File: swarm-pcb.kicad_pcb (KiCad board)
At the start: 4 copper layers, 45 x 40 mm, 120 parts, among them Q301 CJ3139K, U101 USB-TYPE-C-018, U102 2450AT18A100E, U103 ESP32-S3, U104 TS-1187A-B-A-B, U105 TS-1187A-B-A-B, U201 A3901SEJTR-T, U202 ICM-42670-P, U203 NH-B1515RGBA-HF, U205 Motor_1, U206 Motor_2, U301 TLV62569DRL, U302 TP4065, U303 BATT, X101 TZ1269D

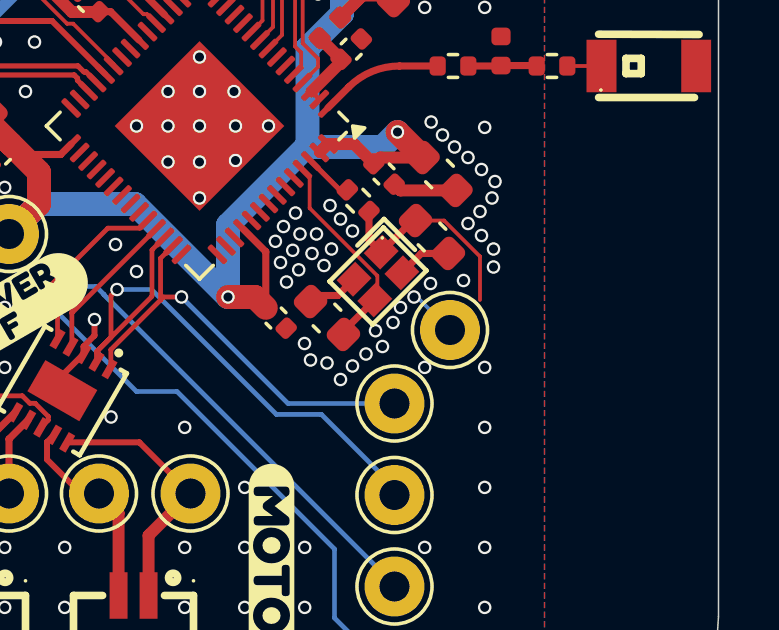
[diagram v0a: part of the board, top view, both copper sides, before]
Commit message: production
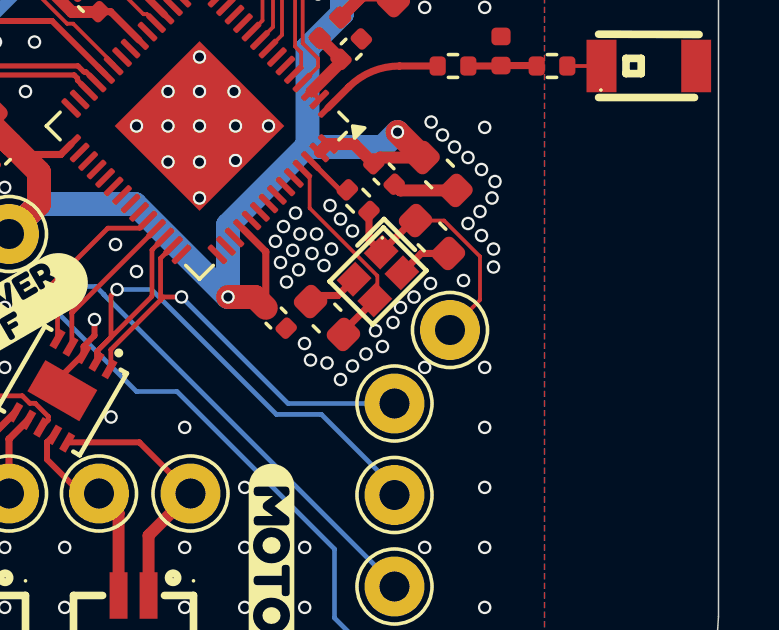
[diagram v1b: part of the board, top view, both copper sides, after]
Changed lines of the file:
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@@
+	)
+	(segment
+		(start 102.05 133.8)
+		(end 103.05 132.8)
+		(width 0.127)
+		(layer "F.Cu")
+		(net 46)
 	)
 	(segment
@@
 		(net 46)
 	)
-	(segment
-		(start 102.05 133.8)
-		(end 101.05 132.8)
-		(width 0.127)
-		(layer "B.Cu")
-		(net 46)
-	)
